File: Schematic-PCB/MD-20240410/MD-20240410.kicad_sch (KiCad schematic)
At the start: 49 parts, among them J1 Conn_01x05_Pin, J2 Conn_01x04_Pin, J3 Conn_01x02_Pin, J4 Conn_01x02_Pin, J5 Conn_01x02_Pin, J6 Conn_01x02_Pin, J7 Conn_01x02_Pin, J8 Conn_01x15_Pin, Q3 NMOS, Q4 NMOS

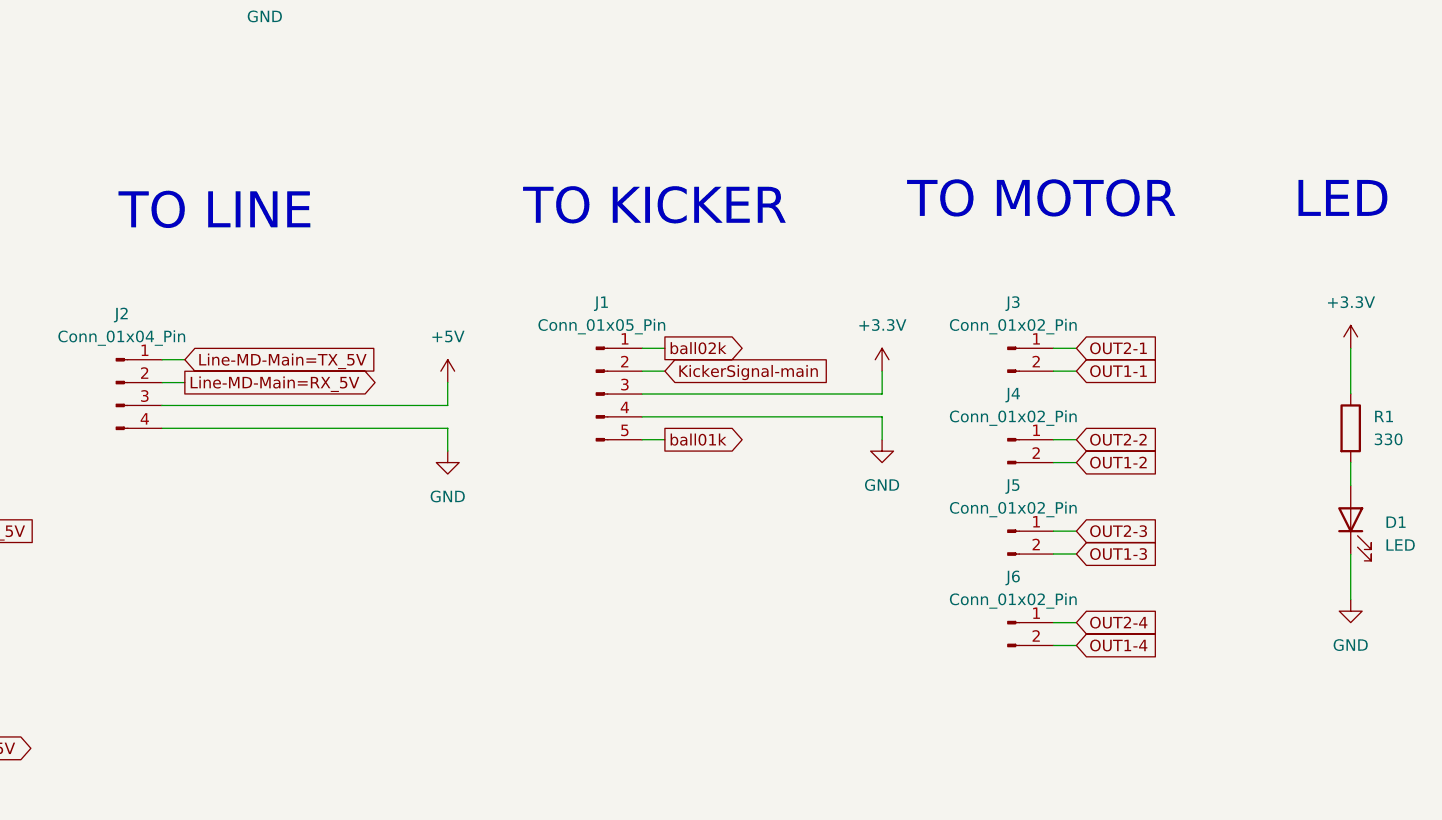
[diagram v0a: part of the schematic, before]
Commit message: MDのDRしたよ
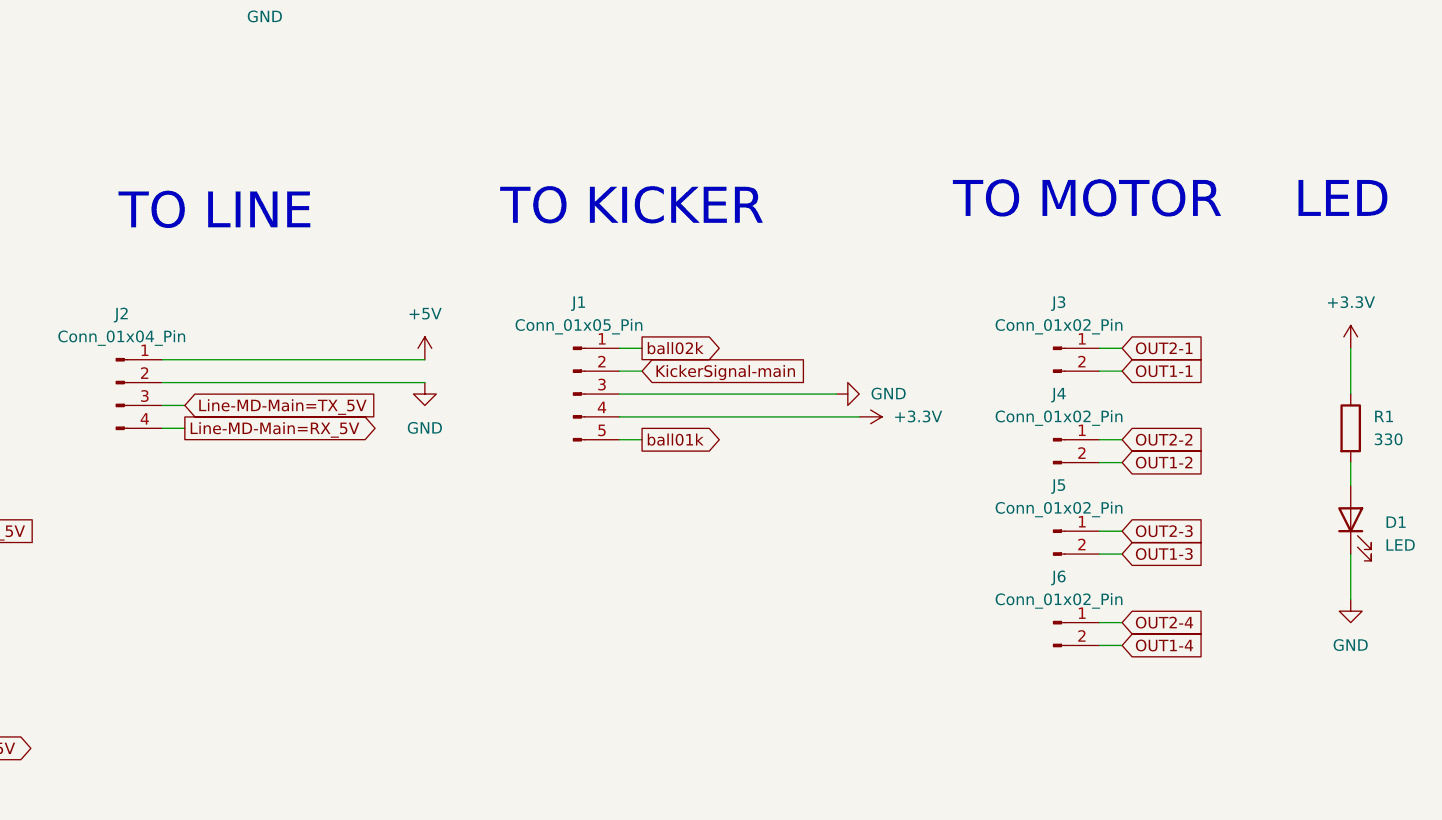
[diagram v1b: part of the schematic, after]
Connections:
- net +3.3V: now also J1.4 (Pin_4); no longer J1.3 (Pin_3)
- net +5V: now also J2.1 (Pin_1); no longer J2.3 (Pin_3)
- net GND: now also J1.3 (Pin_3), J2.2 (Pin_2); no longer J1.4 (Pin_4), J2.4 (Pin_4)
- net Line-MD-Main=RX_5V: now also J2.4 (Pin_4); no longer J2.2 (Pin_2)
- net Line-MD-Main=TX_5V: now also J2.3 (Pin_3); no longer J2.1 (Pin_1)
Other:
- moved on the sheet: J1, J3, J4, J5, J6
